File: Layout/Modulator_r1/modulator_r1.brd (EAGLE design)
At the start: 75.2 x 49.5 mm, 90 parts, among them Q1 FA-20H, U1 ATMEGA328P-AU, U2 TPS79933QDDCRQ1, U3 CC1125RHBT, U4 MCP1700T-3302E/TT, U5 FT232RL, U6 SIP32509DT-T1-GE3

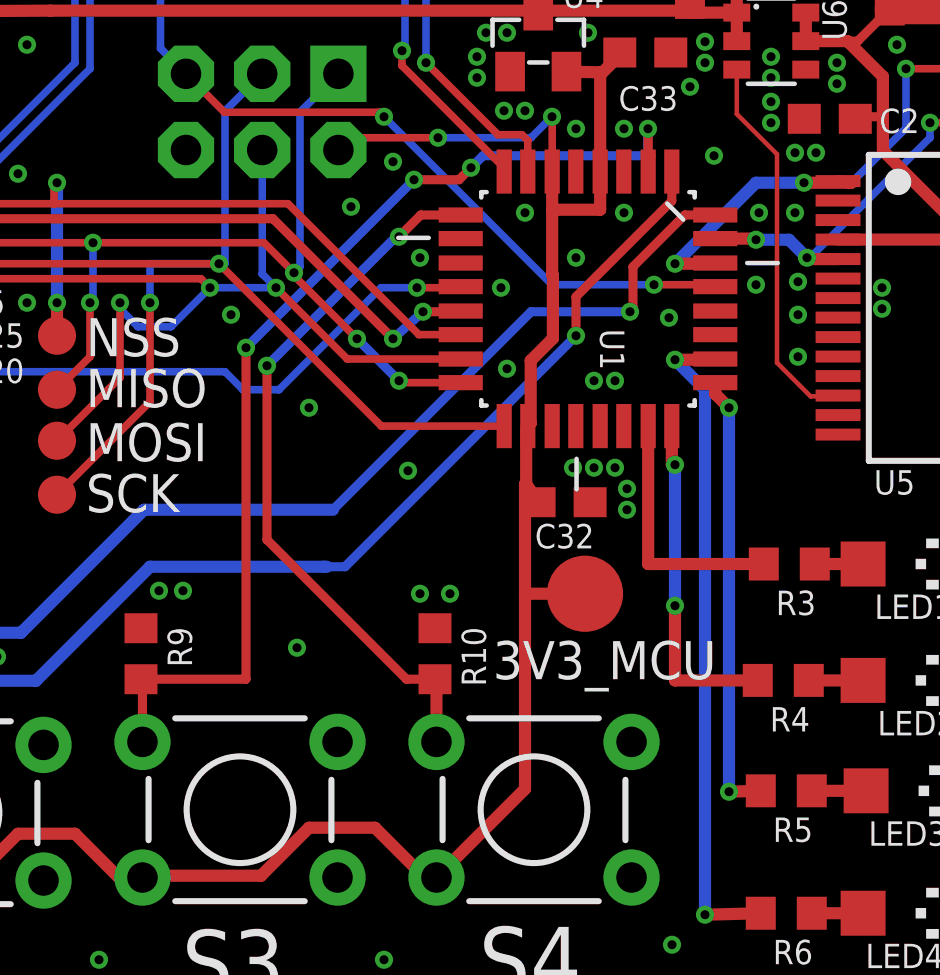
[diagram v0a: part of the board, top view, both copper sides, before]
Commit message: Tweak labels.
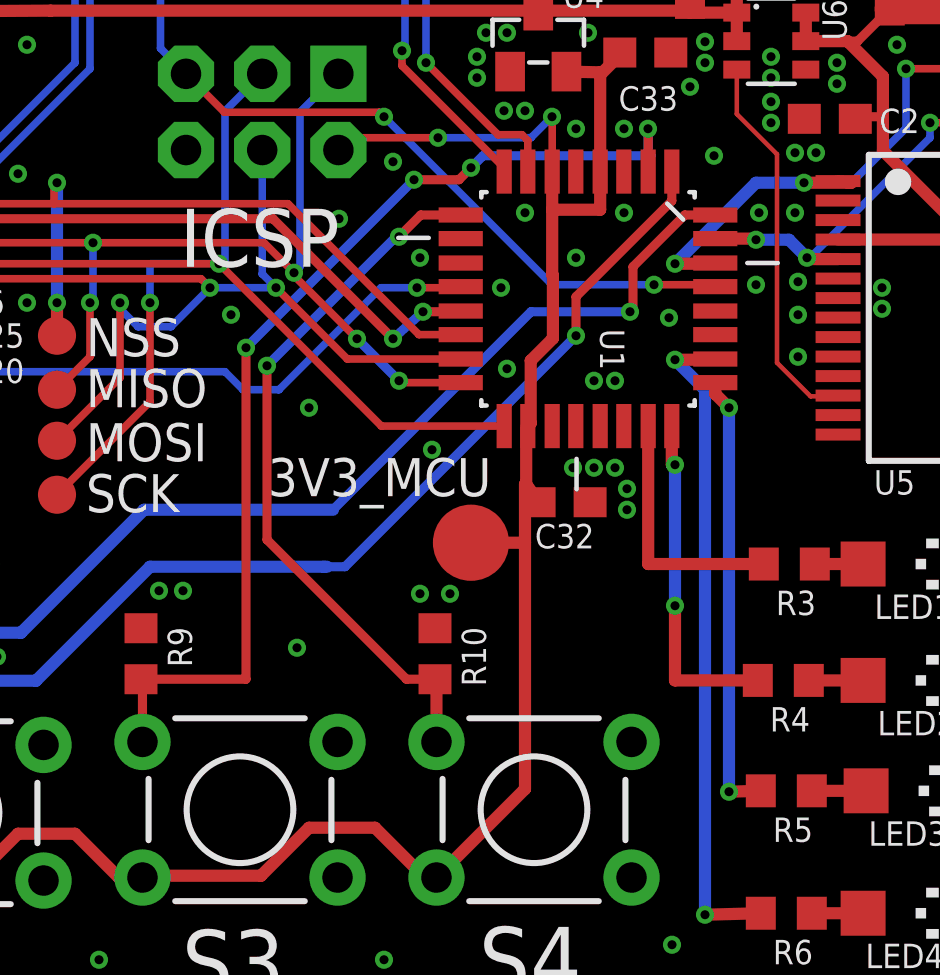
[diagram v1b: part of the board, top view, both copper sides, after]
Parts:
- moved 3V3_MCU 4.16 mm to (44.6, 16.3)
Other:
- board text added: "ICSP"
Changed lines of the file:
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@@
 <text x="62.7" y="2.8" size="2.1844" layer="27">L4</text>
 <text x="13.14" y="42.92" size="1.4224" layer="25" font="vector" ratio="10">r1 - Sept 2015</text>
+<text x="34.9" y="25.5" size="1.9304" layer="25">ICSP</text>
 </plain>
 <attributes>
@@
 <attribute name="TP_SIGNAL_NAME" value="" x="55.4" y="38" size="1.778" layer="27" display="off"/>
 </element>
-<element name="3V3_MCU" library="testpad" package="B2,54" value="PTR1B2,54" x="48.4" y="14.6" smashed="yes">
-<attribute name="TP_SIGNAL_NAME" value="" x="47.13" y="11.425" size="1" layer="37"/>
-<attribute name="NAME" x="45.33" y="11.751" size="1.27" layer="25" ratio="10"/>
-<attribute name="VALUE" x="47.13" y="13.203" size="0.0254" layer="27"/>
+<element name="3V3_MCU" library="testpad" package="B2,54" value="PTR1B2,54" x="44.6" y="16.3" smashed="yes">
+<attribute name="TP_SIGNAL_NAME" value="" x="43.33" y="13.125" size="1" layer="37"/>
+<attribute name="NAME" x="37.83" y="17.851" size="1.27" layer="25" ratio="10"/>
+<attribute name="VALUE" x="43.33" y="14.903" size="0.0254" layer="27"/>
 </element>
 <element name="3V3_RF" library="testpad" package="B2,54" value="PTR1B2,54" x="15.1" y="33.9" smashed="yes">
@@
 <via x="45.8" y="22.1" extent="1-16" drill="0.3"/>
 <via x="42.9" y="25.8" extent="1-16" drill="0.3"/>
-<via x="40.6" y="27.5" extent="1-16" drill="0.3"/>
+<via x="40.2" y="27.1" extent="1-16" drill="0.3"/>
 <via x="42" y="29" extent="1-16" drill="0.3"/>
 <via x="39.2" y="20.8" extent="1-16" drill="0.3"/>
-<via x="42.5" y="18.7" extent="1-16" drill="0.3"/>
+<via x="43.3" y="19.4" extent="1-16" drill="0.3"/>
 <via x="38.8" y="12.8" extent="1-16" drill="0.3"/>
 <via x="28.8" y="12.5" extent="1-16" drill="0.3"/>
@@
 <contactref element="S4" pad="3"/>
 <wire x1="46.87" y1="17.65" x2="46.4" y2="18.25" width="0.4064" layer="1"/>
-<wire x1="46.4" y1="18.25" x2="46.4" y2="14.6" width="0.4064" layer="1"/>
-<wire x1="46.4" y1="14.6" x2="46.4" y2="8.0906" width="0.4064" layer="1"/>
+<wire x1="46.4" y1="18.25" x2="46.4" y2="16.3" width="0.4064" layer="1"/>
+<wire x1="46.4" y1="16.3" x2="46.4" y2="8.0906" width="0.4064" layer="1"/>
 <wire x1="46.4" y1="8.0906" x2="43.4488" y2="5.1394" width="0.4064" layer="1"/>
 <wire x1="43.4488" y1="5.1394" x2="43.0606" y2="5.1394" width="0.4064" layer="1"/>
@@
 <via x="47.3" y="30.5" extent="1-16" drill="0.3"/>
 <contactref element="3V3_MCU" pad="TP"/>
-<wire x1="48.4" y1="14.6" x2="46.4" y2="14.6" width="0.4064" layer="1"/>
+<wire x1="44.6" y1="16.3" x2="46.4" y2="16.3" width="0.4064" layer="1"/>
 </signal>
 <signal name="UART_TX">
